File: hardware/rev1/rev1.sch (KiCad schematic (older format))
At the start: 42 parts, among them J1 Conn_01x09_Female, J2 RFM9X_header, J3 Conn_01x03_Male, Q1 Q_PNP_BCE, U1 BNO055, U2 MPL3115A2, U3 Teensy3.6, U4 BMI088, U5 ADXL345BCCZ, Y1 Crystal_32kHz768

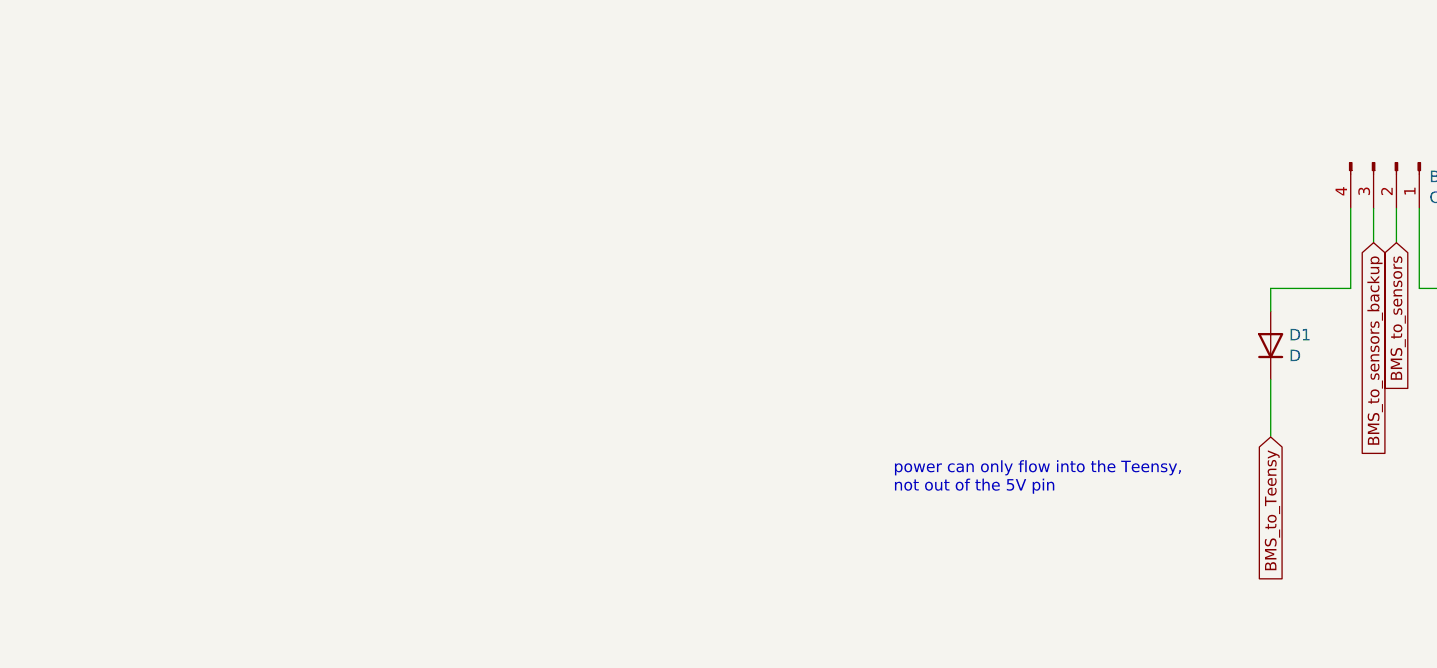
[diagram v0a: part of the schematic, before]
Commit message: wip
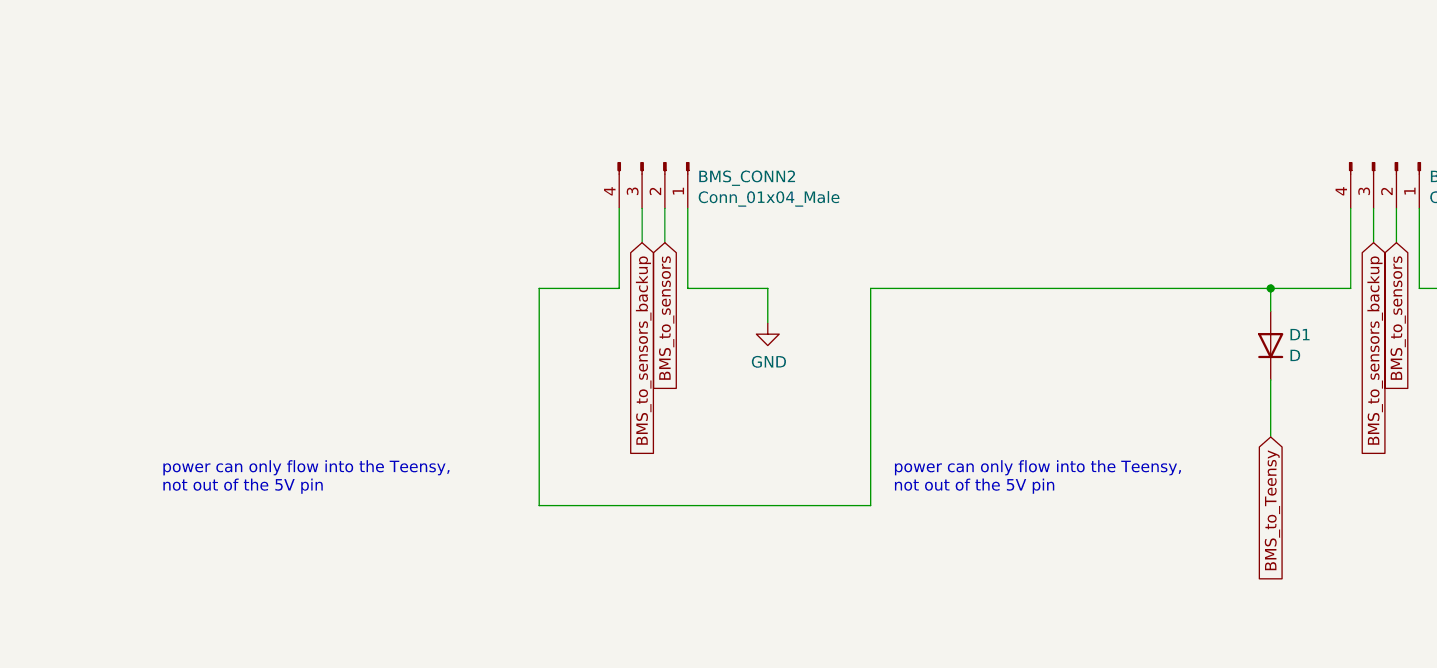
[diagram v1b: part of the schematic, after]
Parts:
- added BMS_CONN2: Conn_01x04_Male, Connector_PinHeader_2.54mm:PinHeader_1x04_P2.54mm_Vertical, symbol Connector:Conn_01x04_Male
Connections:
- net BMS_to_sensors: now also BMS_CONN2.2 (Pin_2)
- net BMS_to_sensors_backup: now also BMS_CONN2.3 (Pin_3)
- net GND: now also BMS_CONN2.1 (Pin_1)
- net at BMS_CONN1.4 (Pin_4), D1.2 (A): now also BMS_CONN2.4 (Pin_4)
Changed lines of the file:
@@
 3.3V_TEENSY
 NoConn ~ 29450 11150
-$Comp
-L Device:D D1
-U 1 1 60275618
-P 24650 11450
-F 0 "D1" V 24696 11370 50  0000 R CNN
-F 1 "D" V 24605 11370 50  0000 R CNN
-F 2 "footprints:D_0805_OEM" H 24650 11450 50  0001 C CNN
-F 3 "~" H 24650 11450 50  0001 C CNN
-	1    24650 11450
-	0    -1   -1   0
-$EndComp
-Text Notes 23000 12100 0    50   ~ 0
-power can only flow into the Teensy,\nnot out of the 5V pin
 NoConn ~ 17800 15400
 Wire Wire Line
@@
 Text Notes 28500 5850 0    50   ~ 0
 TX\n\nRX
-$Comp
-L Connector:Conn_01x04_Male BMS_CONN1
-U 1 1 602BDAB1
-P 25200 10650
-F 0 "BMS_CONN1" V 25262 10794 50  0000 L CNN
-F 1 "Conn_01x04_Male" V 25353 10794 50  0000 L CNN
-F 2 "Connector_PinHeader_2.54mm:PinHeader_1x04_P2.54mm_Vertical" H 25200 10650 50  0001 C CNN
-F 3 "~" H 25200 10650 50  0001 C CNN
-	1    25200 10650
-	0    1    1    0
-$EndComp
-$Comp
-L power:GND #PWR04
-U 1 1 602C00BA
-P 25650 11350
-F 0 "#PWR04" H 25650 11100 50  0001 C CNN
-F 1 "GND" H 25655 11177 50  0000 C CNN
-F 2 "" H 25650 11350 50  0001 C CNN
-F 3 "" H 25650 11350 50  0001 C CNN
-	1    25650 11350
-	1    0    0    -1
-$EndComp
-Text GLabel 24650 11850 3    50   Input ~ 0
-BMS_to_Teensy
-Wire Wire Line
-	25200 10850 25200 11000
-Wire Wire Line
-	25100 10850 25100 11000
-Text GLabel 25100 11000 3    50   Input ~ 0
-BMS_to_sensors_backup
-Text GLabel 25200 11000 3    50   Input ~ 0
-BMS_to_sensors
 Text Notes 25800 5800 0    50   ~ 0
 (GPS) RX -> TX (Teensy)\n(GPS) TX -> RX (Teensy)\n
@@
 Text GLabel 29700 6300 2    50   Input ~ 0
 BMS_to_Teensy
-Wire Wire Line
-	24650 11850 24650 11600
-Wire Wire Line
-	25000 11200 24650 11200
-Wire Wire Line
-	24650 11200 24650 11300
-Wire Wire Line
-	25000 10850 25000 11200
-Wire Wire Line
-	25300 10850 25300 11200
-Wire Wire Line
-	25300 11200 25650 11200
-Wire Wire Line
-	25650 11350 25650 11200
 $Comp
 L Device:Q_PNP_BCE Q1
@@
 	1    0    0    -1
 $EndComp
+Wire Wire Line
+	25650 11350 25650 11200
+Wire Wire Line
+	25300 11200 25650 11200
+Wire Wire Line
+	25300 10850 25300 11200
+Wire Wire Line
+	25000 10850 25000 11200
+Wire Wire Line
+	24650 11200 24650 11300
+Wire Wire Line
+	25000 11200 24650 11200
+Wire Wire Line
+	24650 11850 24650 11600
+Text GLabel 25200 11000 3    50   Input ~ 0
+BMS_to_sensors
+Text GLabel 25100 11000 3    50   Input ~ 0
+BMS_to_sensors_backup
+Wire Wire Line
+	25100 10850 25100 11000
+Wire Wire Line
+	25200 10850 25200 11000
+Text GLabel 24650 11850 3    50   Input ~ 0
+BMS_to_Teensy
+$Comp
+L power:GND #PWR04
+U 1 1 602C00BA
+P 25650 11350
+F 0 "#PWR04" H 25650 11100 50  0001 C CNN
+F 1 "GND" H 25655 11177 50  0000 C CNN
+F 2 "" H 25650 11350 50  0001 C CNN
+F 3 "" H 25650 11350 50  0001 C CNN
+	1    25650 11350
+	1    0    0    -1
+$EndComp
+$Comp
+L Connector:Conn_01x04_Male BMS_CONN1
+U 1 1 602BDAB1
+P 25200 10650
+F 0 "BMS_CONN1" V 25262 10794 50  0000 L CNN
+F 1 "Conn_01x04_Male" V 25353 10794 50  0000 L CNN
+F 2 "Connector_PinHeader_2.54mm:PinHeader_1x04_P2.54mm_Vertical" H 25200 10650 50  0001 C CNN
+F 3 "~" H 25200 10650 50  0001 C CNN
+	1    25200 10650
+	0    1    1    0
+$EndComp
+Text Notes 23000 12100 0    50   ~ 0
+power can only flow into the Teensy,\nnot out of the 5V pin
+$Comp
+L Device:D D1
+U 1 1 60275618
+P 24650 11450
+F 0 "D1" V 24696 11370 50  0000 R CNN
+F 1 "D" V 24605 11370 50  0000 R CNN
+F 2 "footprints:D_0805_OEM" H 24650 11450 50  0001 C CNN
+F 3 "~" H 24650 11450 50  0001 C CNN
+	1    24650 11450
+	0    -1   -1   0
+$EndComp
+Wire Wire Line
+	22450 11350 22450 11200
+Wire Wire Line
+	22100 11200 22450 11200
+Wire Wire Line
+	22100 10850 22100 11200
+Wire Wire Line
+	21800 10850 21800 11200
+Wire Wire Line
+	21800 11200 21450 11200
+Text GLabel 22000 11000 3    50   Input ~ 0
+BMS_to_sensors
+Text GLabel 21900 11000 3    50   Input ~ 0
+BMS_to_sensors_backup
+Wire Wire Line
+	21900 10850 21900 11000
+Wire Wire Line
+	22000 10850 22000 11000
+$Comp
+L power:GND #PWR015
+U 1 1 6047CFA5
+P 22450 11350
+F 0 "#PWR015" H 22450 11100 50  0001 C CNN
+F 1 "GND" H 22455 11177 50  0000 C CNN
+F 2 "" H 22450 11350 50  0001 C CNN
+F 3 "" H 22450 11350 50  0001 C CNN
+	1    22450 11350
+	1    0    0    -1
+$EndComp
+$Comp
+L Connector:Conn_01x04_Male BMS_CONN2
+U 1 1 6047CFAF
+P 22000 10650
+F 0 "BMS_CONN2" V 22062 10794 50  0000 L CNN
+F 1 "Conn_01x04_Male" V 22153 10794 50  0000 L CNN
+F 2 "Connector_PinHeader_2.54mm:PinHeader_1x04_P2.54mm_Vertical" H 22000 10650 50  0001 C CNN
+F 3 "~" H 22000 10650 50  0001 C CNN
+	1    22000 10650
+	0    1    1    0
+$EndComp
+Text Notes 19800 12100 0    50   ~ 0
+power can only flow into the Teensy,\nnot out of the 5V pin
+Wire Wire Line
+	21450 12150 22900 12150
+Wire Wire Line
+	22900 12150 22900 11200
+Wire Wire Line
+	22900 11200 24650 11200
+Wire Wire Line
+	21450 11200 21450 12150
+Connection ~ 24650 11200
 $EndSCHEMATC
